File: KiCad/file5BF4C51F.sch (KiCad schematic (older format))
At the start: 6 parts, among them J401 CONN_01X06, J402 CONN_01X10, J403 CONN_01X10

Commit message: Changes for FlexFox80
Wholesale changes for new project.
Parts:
- J401: symbol ARDF-2-Band-MiniTx-rescue:CONN_01X06 -> FlexFox80-rescue:CONN_01X06-ARDF-2-Band-MiniTx-rescue
- J402, J403: symbol ARDF-2-Band-MiniTx-rescue:CONN_01X10 -> FlexFox80-rescue:CONN_01X10-ARDF-2-Band-MiniTx-rescue
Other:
- note added: "BOM-ONLY: Flex Fox 80 ARDF Transmitter"
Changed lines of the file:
@@
 $EndComp
 $Comp
-L ARDF-2-Band-MiniTx-rescue:CONN_01X06 J401
+L FlexFox80-rescue:CONN_01X06-ARDF-2-Band-MiniTx-rescue J401
 U 1 1 5C10B0E5
 P 3100 3700
@@
 $EndComp
 $Comp
-L ARDF-2-Band-MiniTx-rescue:CONN_01X10 J402
+L FlexFox80-rescue:CONN_01X10-ARDF-2-Band-MiniTx-rescue J402
 U 1 1 5C10B110
 P 3750 3850
@@
 $EndComp
 $Comp
-L ARDF-2-Band-MiniTx-rescue:CONN_01X10 J403
+L FlexFox80-rescue:CONN_01X10-ARDF-2-Band-MiniTx-rescue J403
 U 1 1 5C10B14B
 P 4250 3850
@@
 Text Notes 2900 3250 0    61   ~ 12
 Header sockets for Huzzah board
+Text Notes 7200 6750 0    118  ~ 24
+BOM-ONLY: Flex Fox 80 ARDF Transmitter
 $EndSCHEMATC

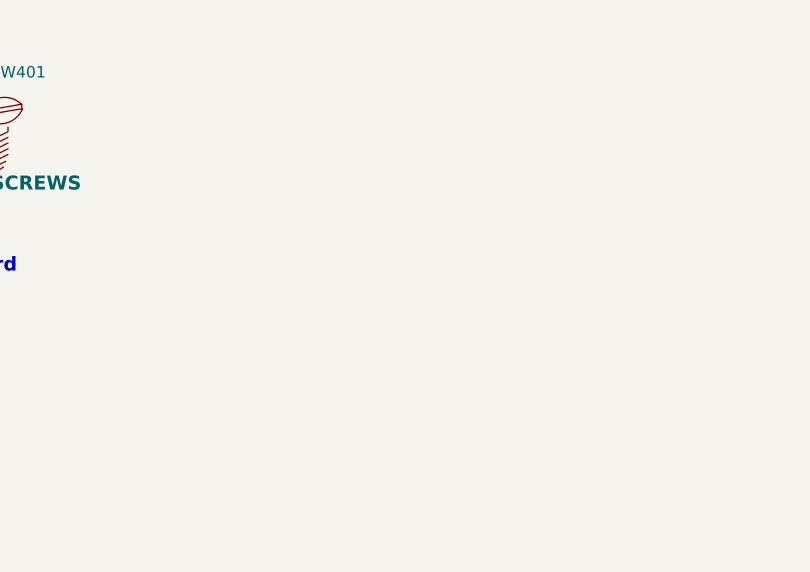
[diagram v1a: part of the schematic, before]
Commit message: Updates to Schematic
Updates to Schematic
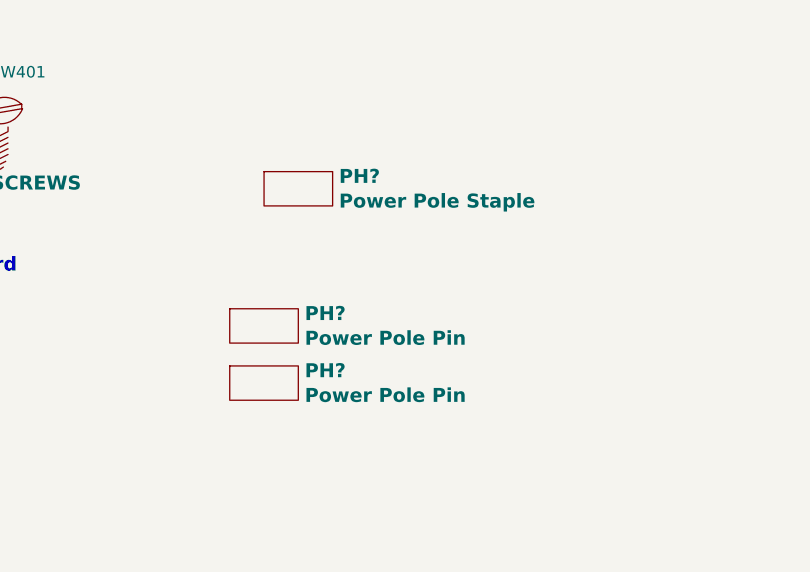
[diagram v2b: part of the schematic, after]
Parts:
- added PH?: Power Pole Staple, symbol Device:PinlessHardware
- added PH? (x2): Power Pole Pin, symbol Device:PinlessHardware
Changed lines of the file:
@@
 Text Notes 7200 6750 0    118  ~ 24
 BOM-ONLY: Flex Fox 80 ARDF Transmitter
+$Comp
+L Device:PinlessHardware PH?
+U 1 1 607EA3F6
+P 5700 3000
+F 0 "PH?" H 5878 3179 61  0000 L CNB
+F 1 "Power Pole Staple" H 5878 3071 61  0000 L CNB
+F 2 "" H 5700 3000 39  0001 C CNN
+F 3 "" H 5700 3000 39  0001 C CNN
+F 4 "2243-114555P2-ND" H 5700 3000 50  0001 C CNN "Part No."
+F 5 "<a href=\"https://www.digikey.com/products/en?keywords=2243-114555P2-ND\">Link</a>" H 5700 3000 50  0001 C CNN "Link"
+F 6 "TH" H 5700 3000 50  0001 C CNN "Manufacturer"
+F 7 "TH" H 5700 3000 50  0001 C CNN "Manufacturer PN"
+F 8 "TH" H 5700 3000 50  0001 C CNN "Description"
+	1    5700 3000
+	1    0    0    -1
+$EndComp
+$Comp
+L Device:PinlessHardware PH?
+U 1 1 607EC98E
+P 5550 3600
+F 0 "PH?" H 5728 3779 61  0000 L CNB
+F 1 "Power Pole Pin" H 5728 3671 61  0000 L CNB
+F 2 "" H 5550 3600 39  0001 C CNN
+F 3 "" H 5550 3600 39  0001 C CNN
+F 4 "2243-1377G2-BK-ND" H 5550 3600 50  0001 C CNN "Part No."
+F 5 "<a href=\"https://www.digikey.com/products/en?keywords=2243-1377G2-BK-ND\">Link</a>" H 5550 3600 50  0001 C CNN "Link"
+F 6 "TH" H 5550 3600 50  0001 C CNN "Manufacturer"
+F 7 "TH" H 5550 3600 50  0001 C CNN "Manufacturer PN"
+F 8 "TH" H 5550 3600 50  0001 C CNN "Description"
+	1    5550 3600
+	1    0    0    -1
+$EndComp
+$Comp
+L Device:PinlessHardware PH?
+U 1 1 607ED223
+P 5550 3850
+F 0 "PH?" H 5728 4029 61  0000 L CNB
+F 1 "Power Pole Pin" H 5728 3921 61  0000 L CNB
+F 2 "" H 5550 3850 39  0001 C CNN
+F 3 "" H 5550 3850 39  0001 C CNN
+F 4 "2243-1377G2-BK-ND" H 5550 3850 50  0001 C CNN "Part No."
+F 5 "<a href=\"https://www.digikey.com/products/en?keywords=2243-1377G2-BK-ND\">Link</a>" H 5550 3850 50  0001 C CNN "Link"
+F 6 "TH" H 5550 3850 50  0001 C CNN "Manufacturer"
+F 7 "TH" H 5550 3850 50  0001 C CNN "Manufacturer PN"
+F 8 "TH" H 5550 3850 50  0001 C CNN "Description"
+	1    5550 3850
+	1    0    0    -1
+$EndComp
 $EndSCHEMATC
